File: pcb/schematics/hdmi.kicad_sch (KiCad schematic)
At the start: 19 parts

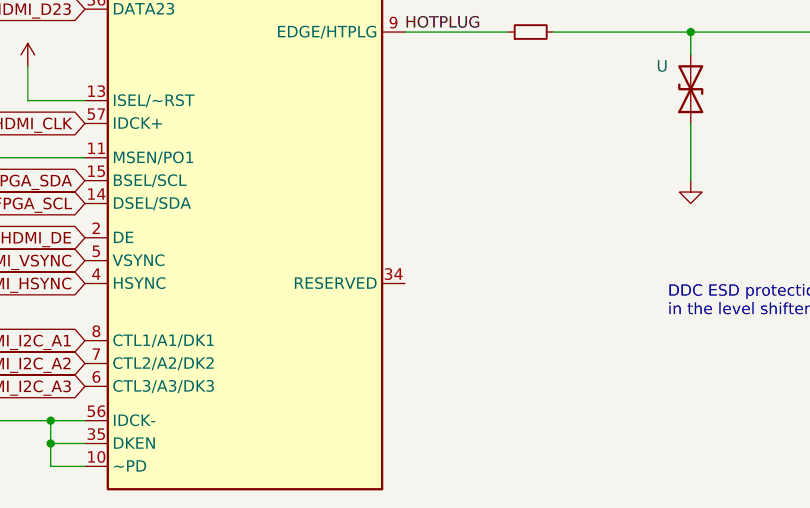
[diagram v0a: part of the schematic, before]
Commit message: passed erc and drc
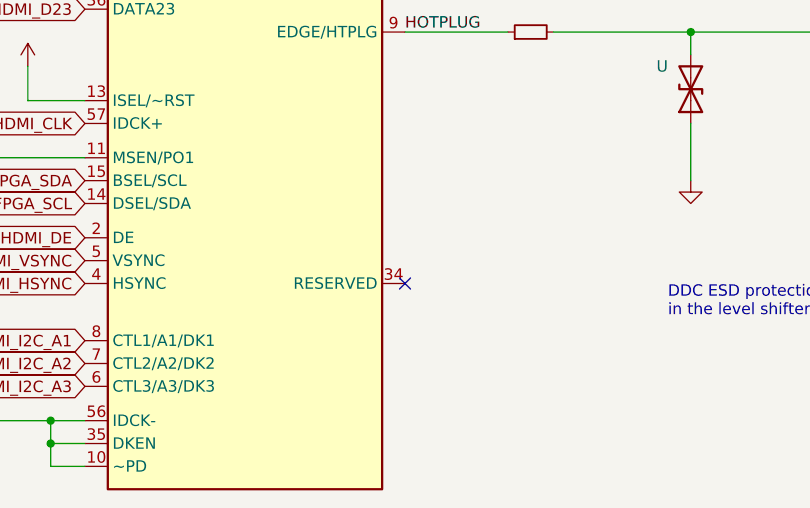
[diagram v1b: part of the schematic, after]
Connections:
- no-connect marks 2 -> 3
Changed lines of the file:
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@@
   (no_connect (at 171.45 113.03))
   (no_connect (at 171.45 125.73))
+  (no_connect (at 125.73 156.21))
   (wire (pts (xy 135.89 110.49) (xy 135.89 102.87))
     (stroke (width 0) (type default))
